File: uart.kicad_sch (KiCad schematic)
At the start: 10 parts, among them U7 MCP2200-I-SO, X1 12M

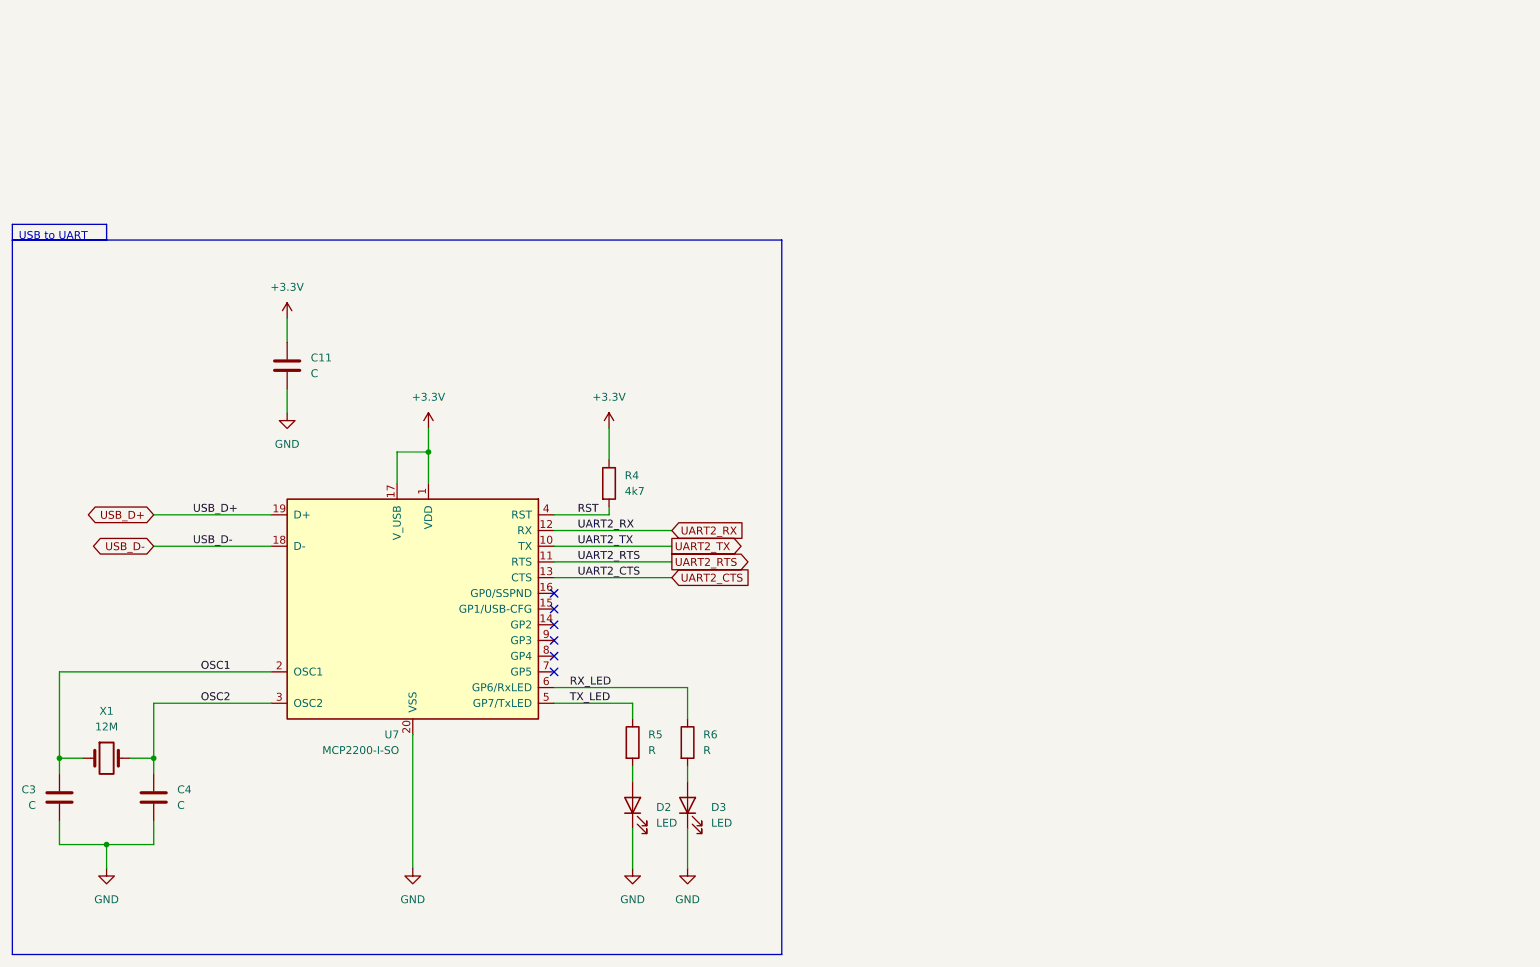
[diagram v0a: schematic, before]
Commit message: asdfsa
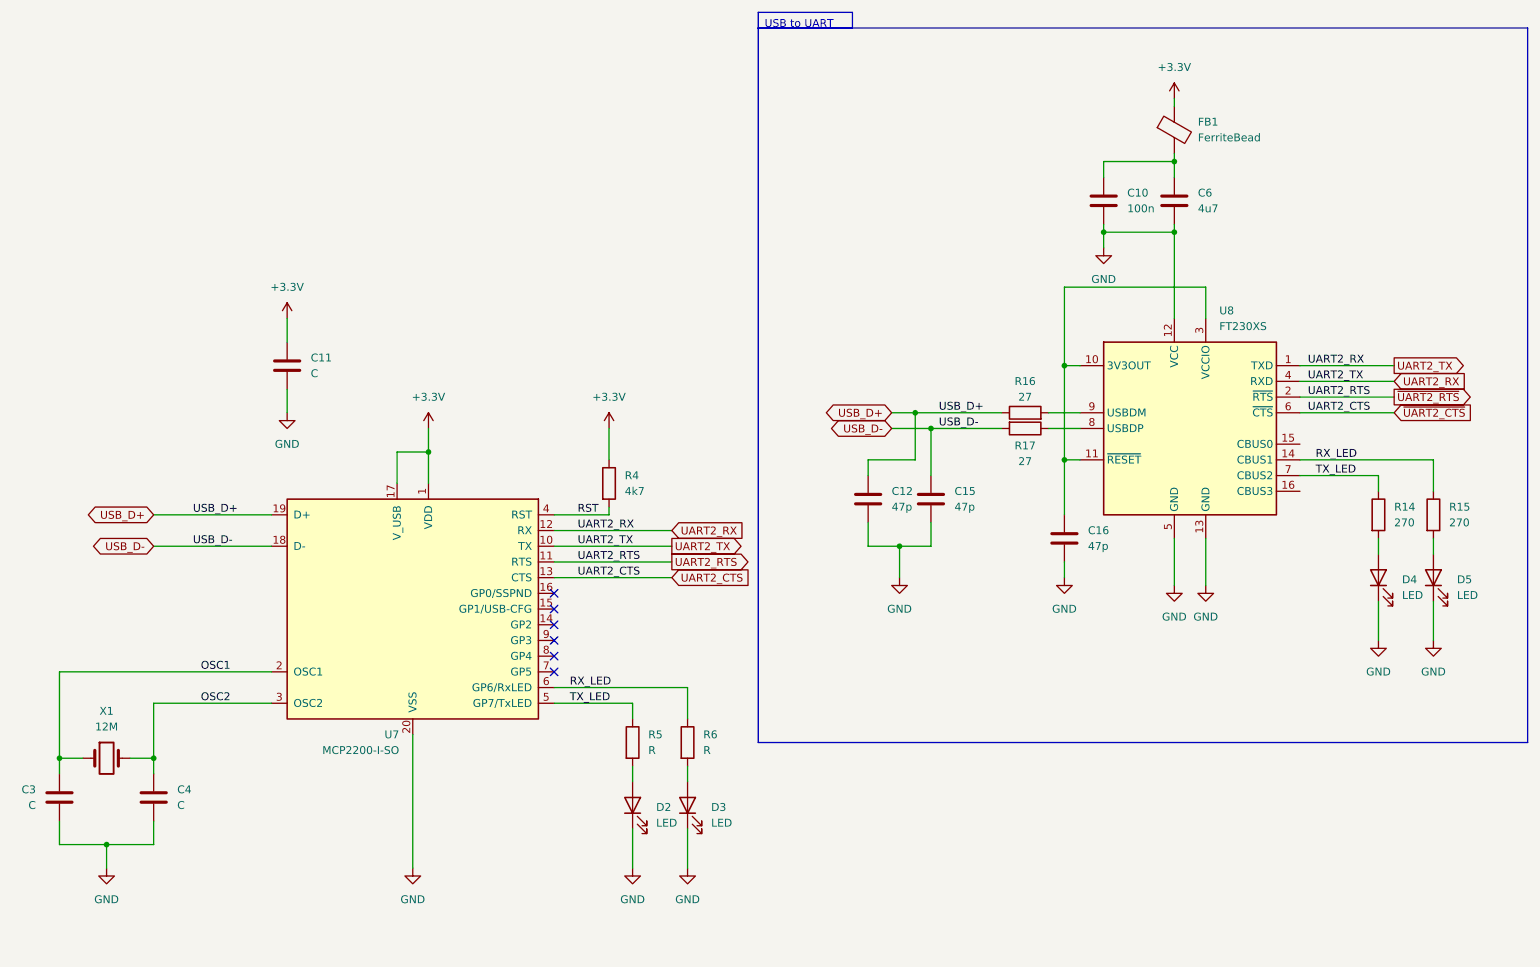
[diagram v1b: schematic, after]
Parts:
- added C10: 100n, Capacitor_SMD:C_0603_1608Metric, symbol Device:C
- added C12, C15, C16: 47p, Capacitor_SMD:C_0603_1608Metric, symbol Device:C
- added C6: 4u7, Capacitor_SMD:C_0603_1608Metric, symbol Device:C
- added D4, D5: LED, LED_SMD:LED_PLCC-2_3x2mm_AK, symbol Device:LED
- added FB1: FerriteBead, Capacitor_SMD:C_0603_1608Metric, symbol Device:FerriteBead
- added R14, R15: 270, Resistor_SMD:R_0603_1608Metric, symbol Device:R
- added R16, R17: 27, Resistor_SMD:R_0603_1608Metric, symbol Device:R
- added U8: FT230XS, Package_SO:SSOP-16_3.9x4.9mm_P0.635mm, symbol Interface_USB:FT230XS
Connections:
- net UART2_TX is gone; now on net UART2_RX: U7.10 (TX)
- net +3.3V: now also FB1.1
- net GND: now also C10.2, C12.2, C15.2, C16.2, C6.2, D4.1 (K), D5.1 (K), U8.12 (VCC), U8.13 (GND), U8.5 (GND)
- net RX_LED: now also R15.1, U8.14 (CBUS1)
- net TX_LED: now also R14.1, U8.7 (CBUS2)
- net UART2_CTS: now also U8.6 (~{CTS})
- net UART2_RTS: now also U8.2 (~{RTS})
- net UART2_RX: now also U8.1 (TXD), U8.4 (RXD)
- net USB_D+: now also C12.1, R16.1
- net USB_D-: now also C15.1, R17.2
- new net: R17.1, U8.8 (USBDP)
- new net: D5.2 (A), R15.2
- new net: C16.1, U8.10 (3V3OUT), U8.11 (~{RESET}), U8.3 (VCCIO)
- new net: D4.2 (A), R14.2
- new net: R16.2, U8.9 (USBDM)
- new net: C10.1, C6.1, FB1.2

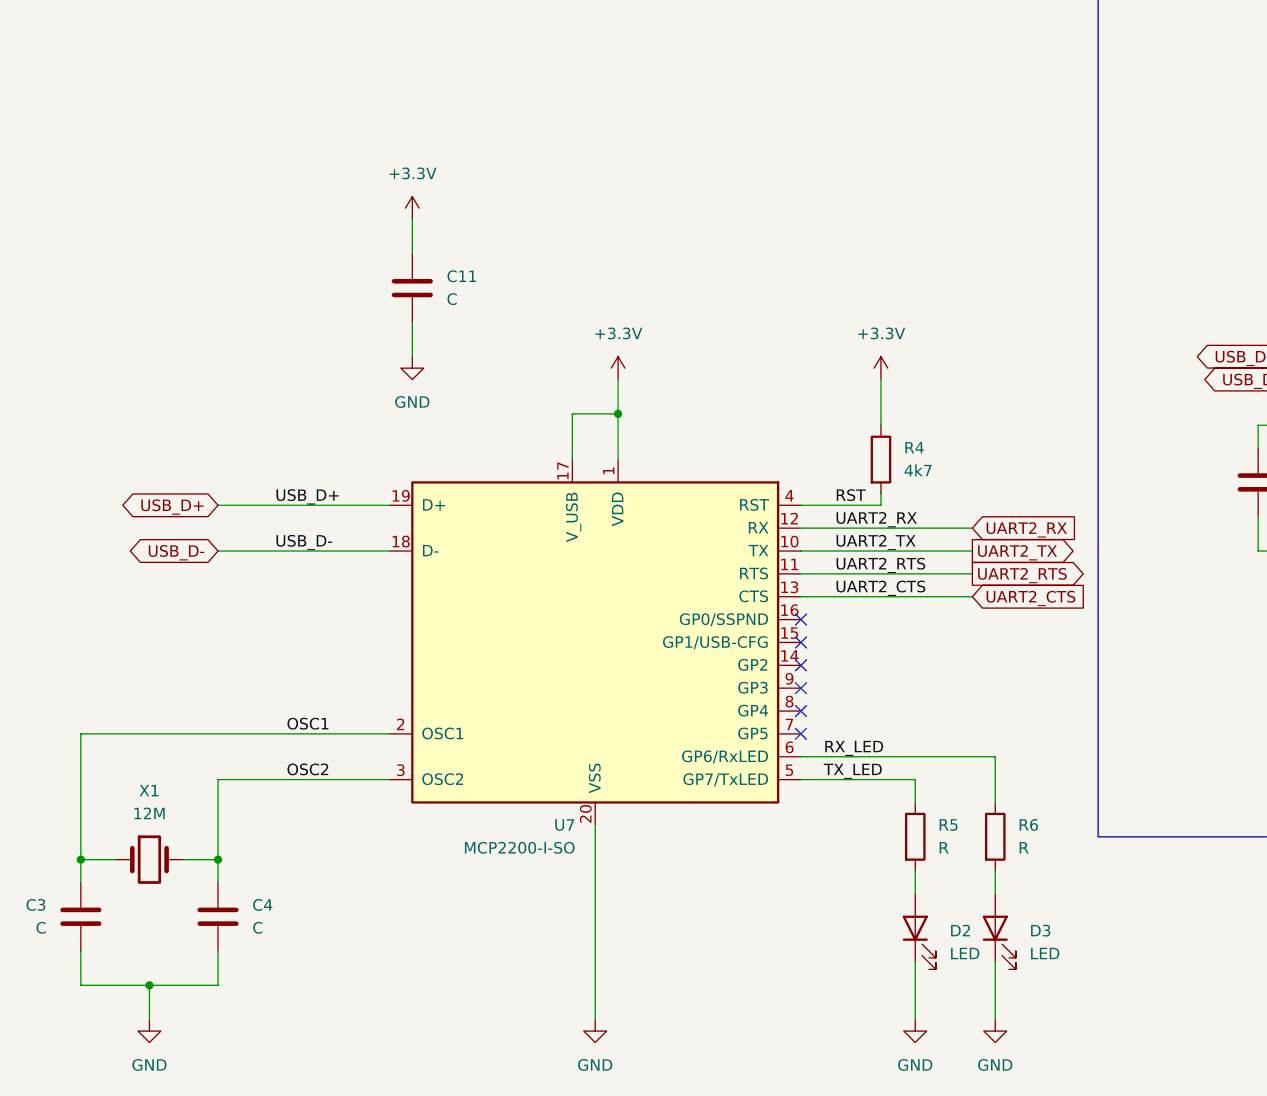
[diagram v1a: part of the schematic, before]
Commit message: asdfsa
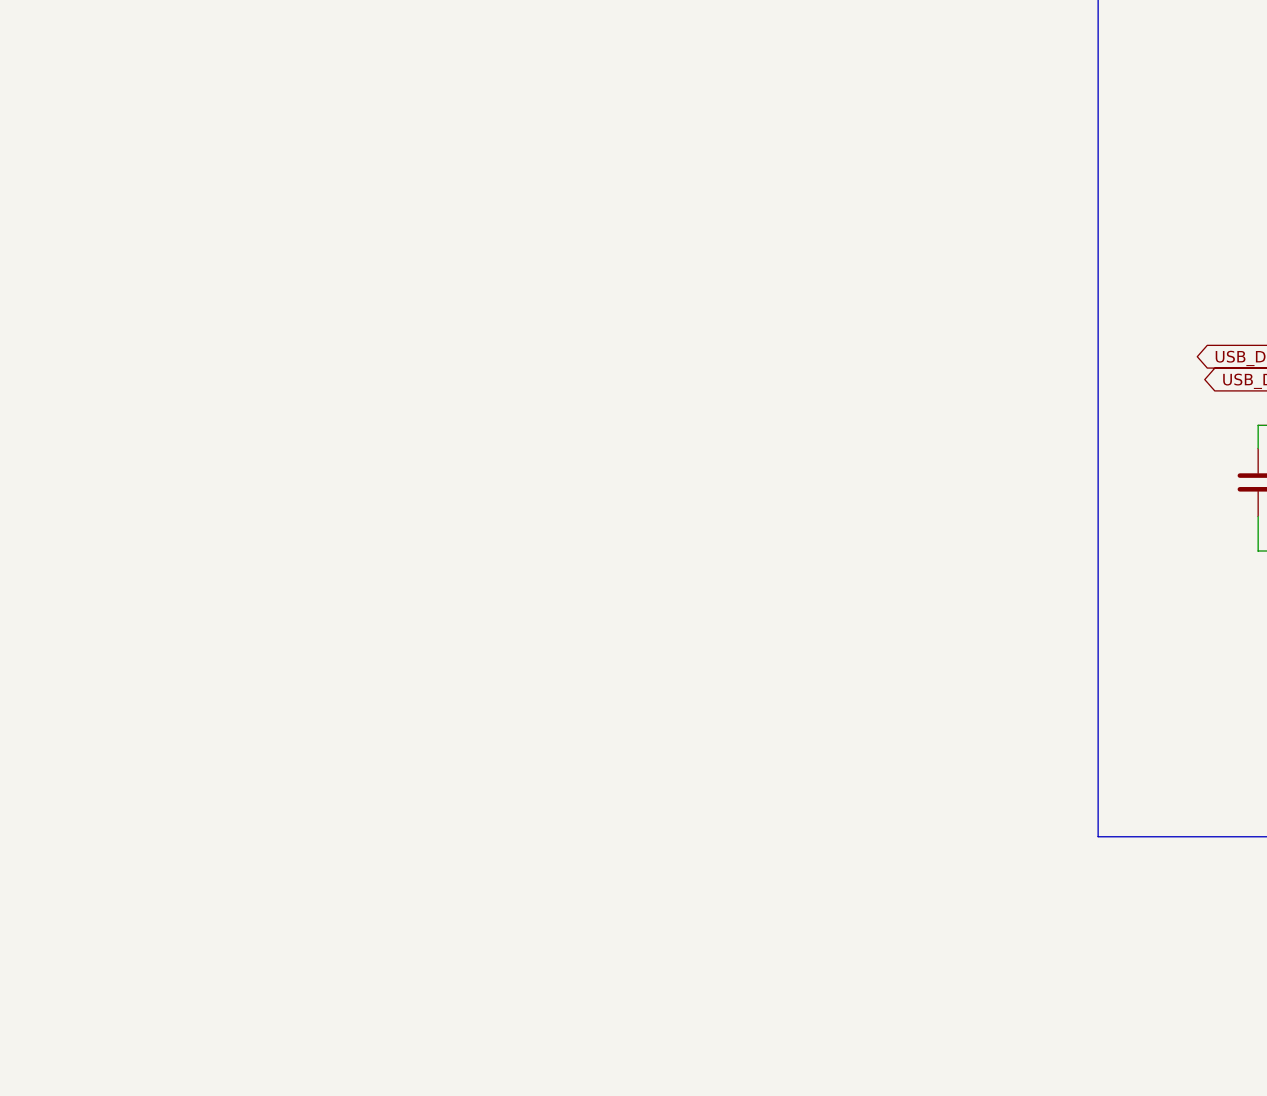
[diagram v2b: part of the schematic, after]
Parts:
- removed C11, C3, C4: C, Capacitor_SMD:C_0603_1608Metric, symbol Device:C
- removed D2, D3: LED, LED_SMD:LED_PLCC-2_3x2mm_AK, symbol Device:LED
- removed R4: 4k7, Resistor_SMD:R_0603_1608Metric, symbol Device:R
- removed R5, R6: R, Resistor_SMD:R_0603_1608Metric, symbol Device:R
- removed U7: MCP2200-I-SO, Package_SO:SOIC-20W_7.5x12.8mm_P1.27mm, symbol Interface_USB:MCP2200-I-SO
- removed X1: 12M, custom:73-XT49M1200-S, symbol Device:Crystal
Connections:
- net UART2_CTS renamed ~{UART2_CTS}
- net UART2_RTS renamed ~{UART2_RTS}
- no-connect marks 6 -> 0
